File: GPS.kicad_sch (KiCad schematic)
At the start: 18 parts, among them J11 GPS_I2C, J2 RFPC-SMA28-F, SW4 GPS_RESET, U9 PA1616S_GPS

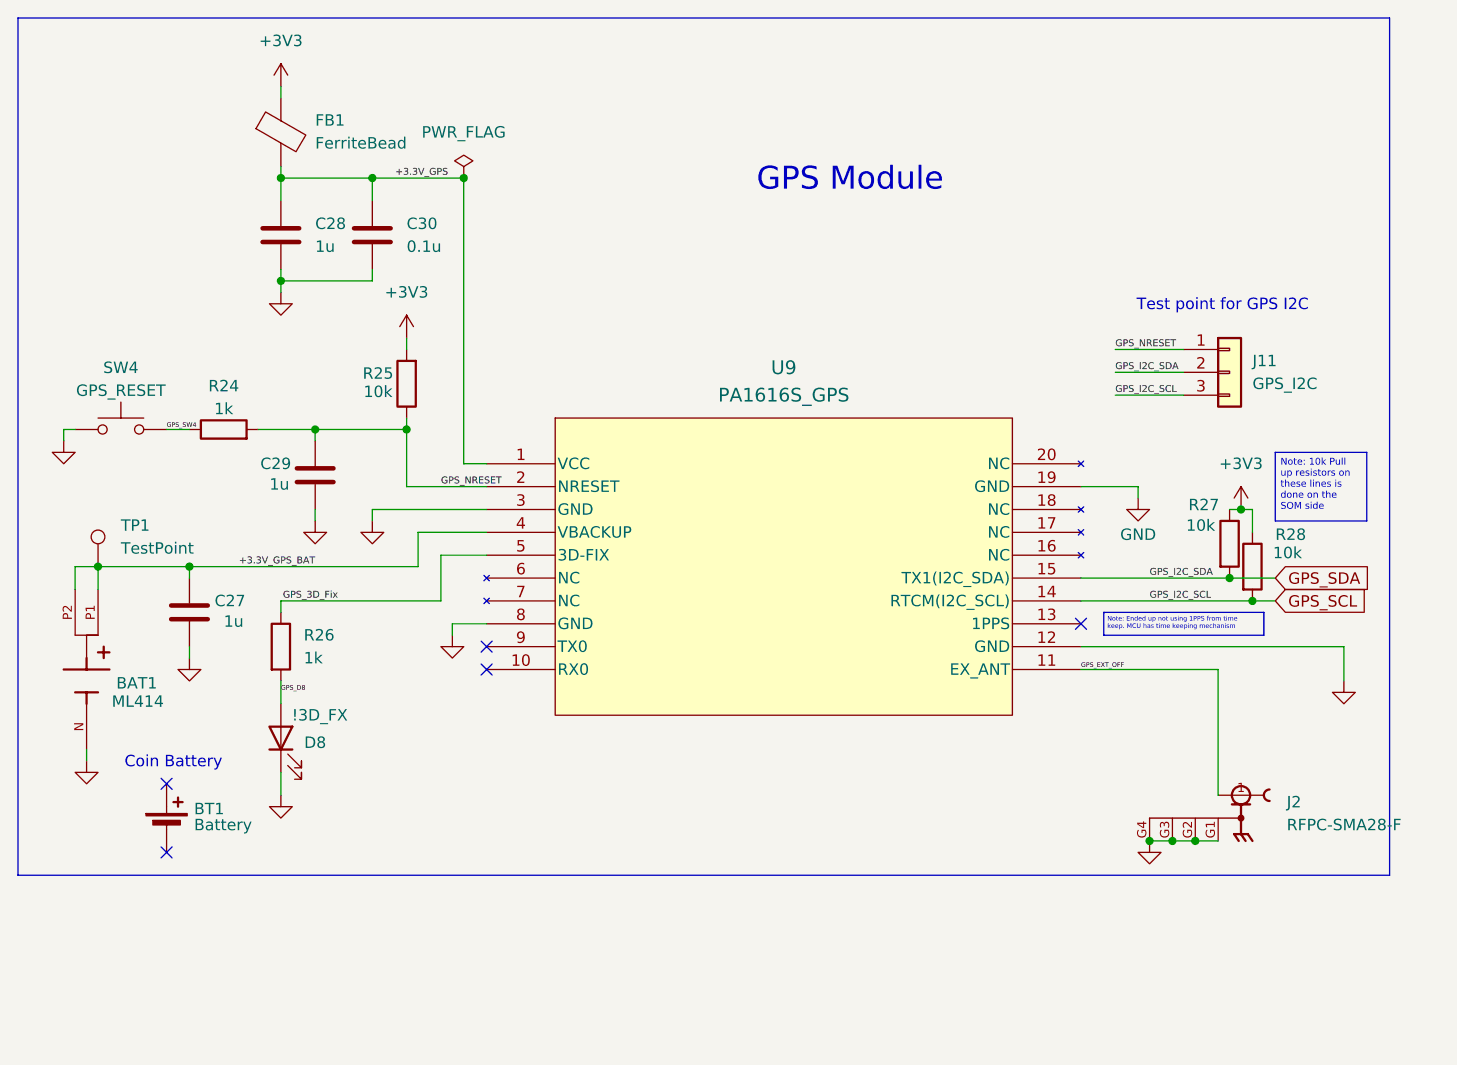
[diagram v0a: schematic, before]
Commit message: done antenna
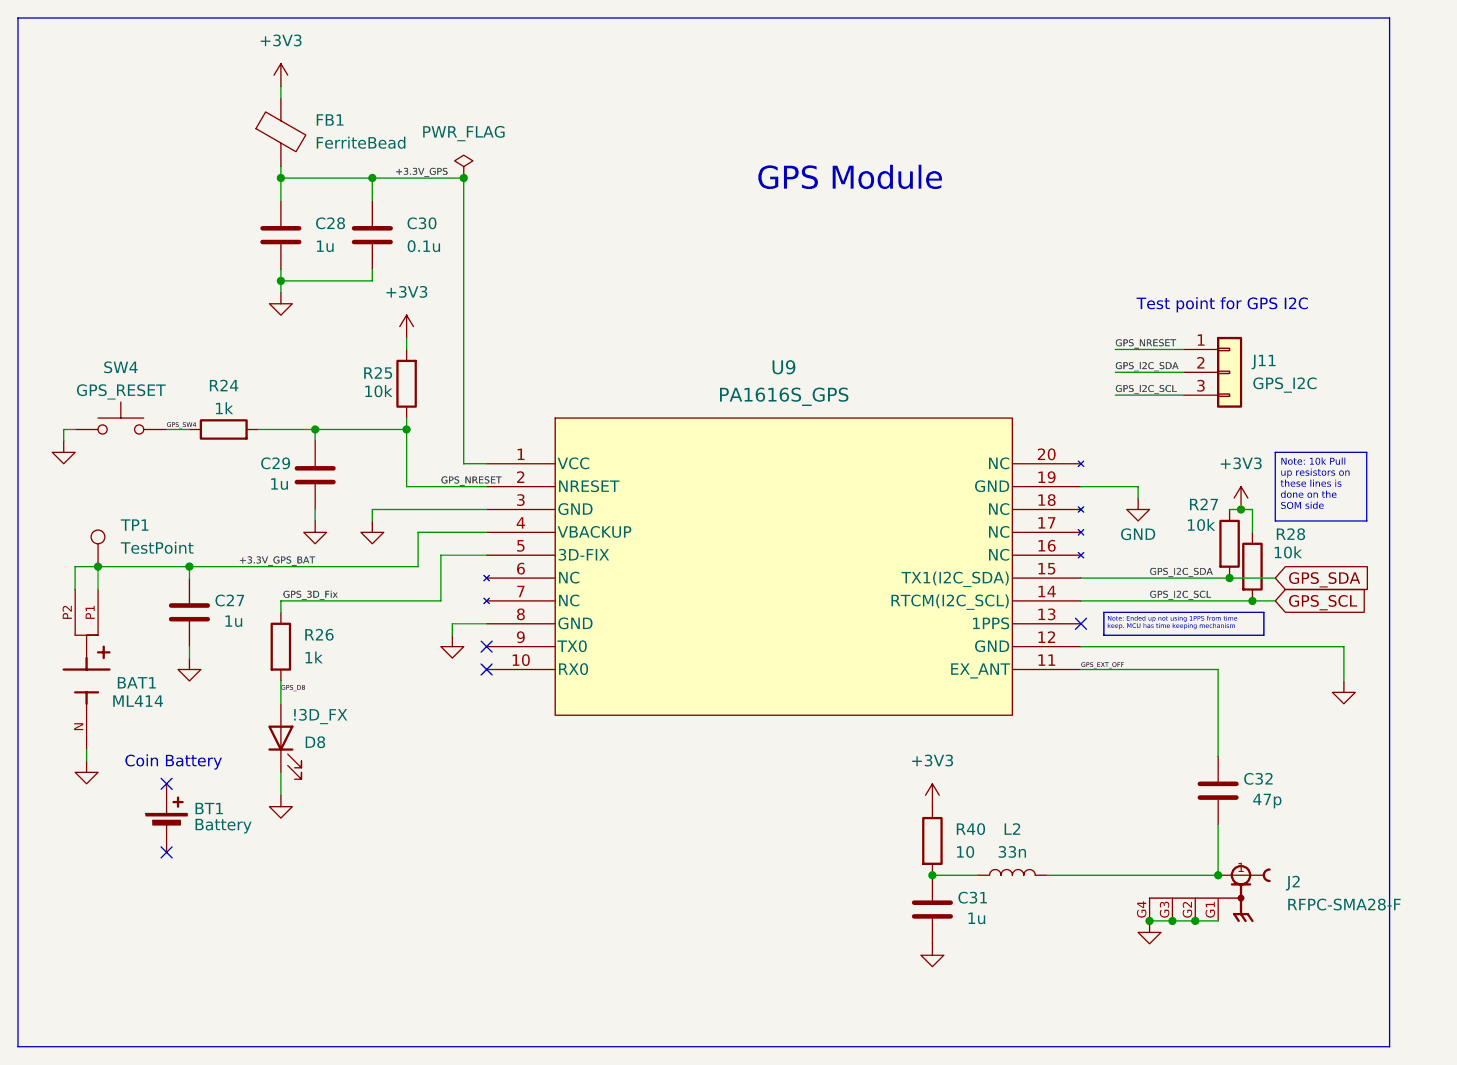
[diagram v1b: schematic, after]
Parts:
- added C31: 1u, Capacitor_SMD:C_0603_1608Metric_Pad1.08x0.95mm_HandSolder, symbol Device:C
- added C32: 47p, Capacitor_SMD:C_0603_1608Metric_Pad1.08x0.95mm_HandSolder, symbol Device:C
- added L2: 33n, Inductor_SMD:L_0603_1608Metric_Pad1.05x0.95mm_HandSolder, symbol Device:L
- added R40: 10, Resistor_SMD:R_0603_1608Metric_Pad0.98x0.95mm_HandSolder, symbol Device:R
- J2: footprint RFPC-SMA28-F:GRADCONN_RFPC-SMA28-F -> TSOM Lib:GRADCONN_RFPC-SMA28-F
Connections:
- net +3V3: now also R40.1
- net GND: now also C31.2
- net GPS_EXT_OFF: now also C32.1; no longer J2.1
- new net: C31.1, L2.1, R40.2
- new net: C32.2, J2.1, L2.2
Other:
- moved on the sheet: J2
